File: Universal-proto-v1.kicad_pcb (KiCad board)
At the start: 2 copper layers, 2 parts, among them J1 Bus_ISA_8bit, U1 RP2350B

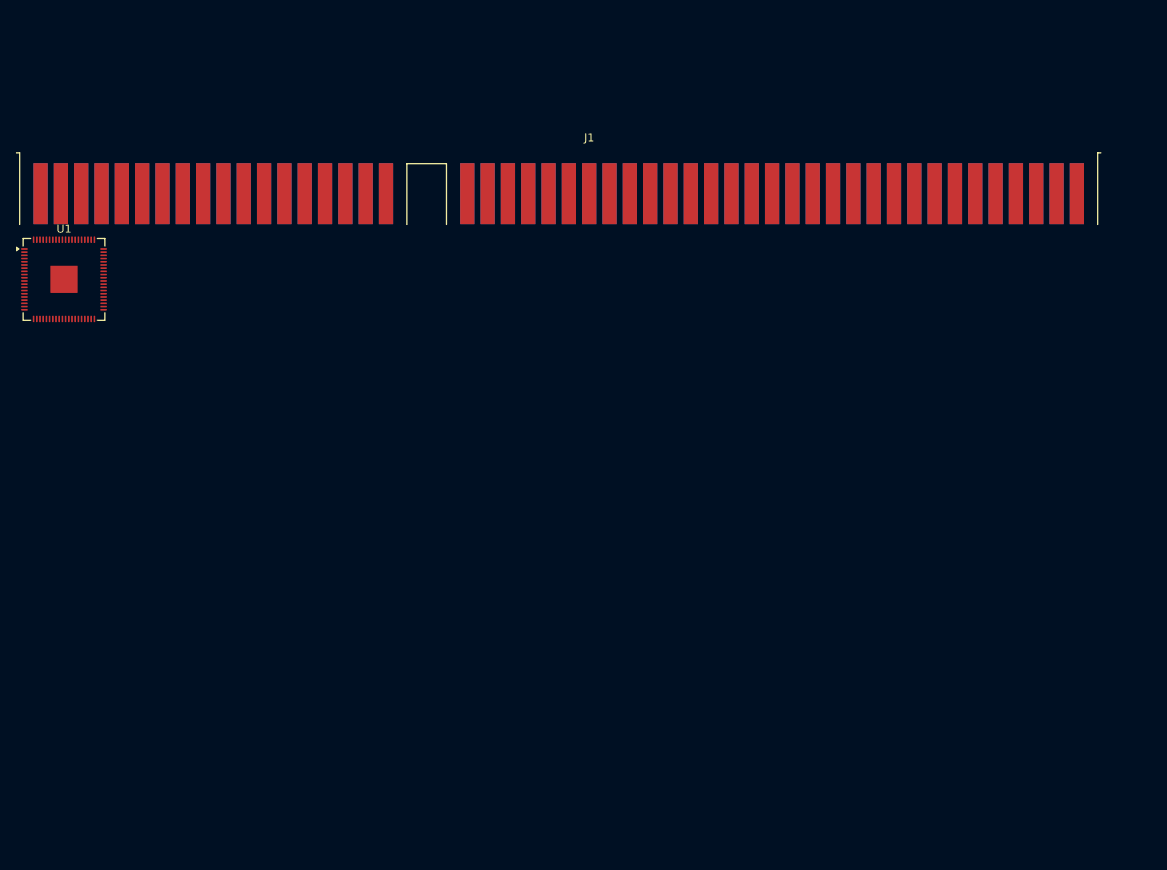
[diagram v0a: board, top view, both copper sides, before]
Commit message: Start work on PCB
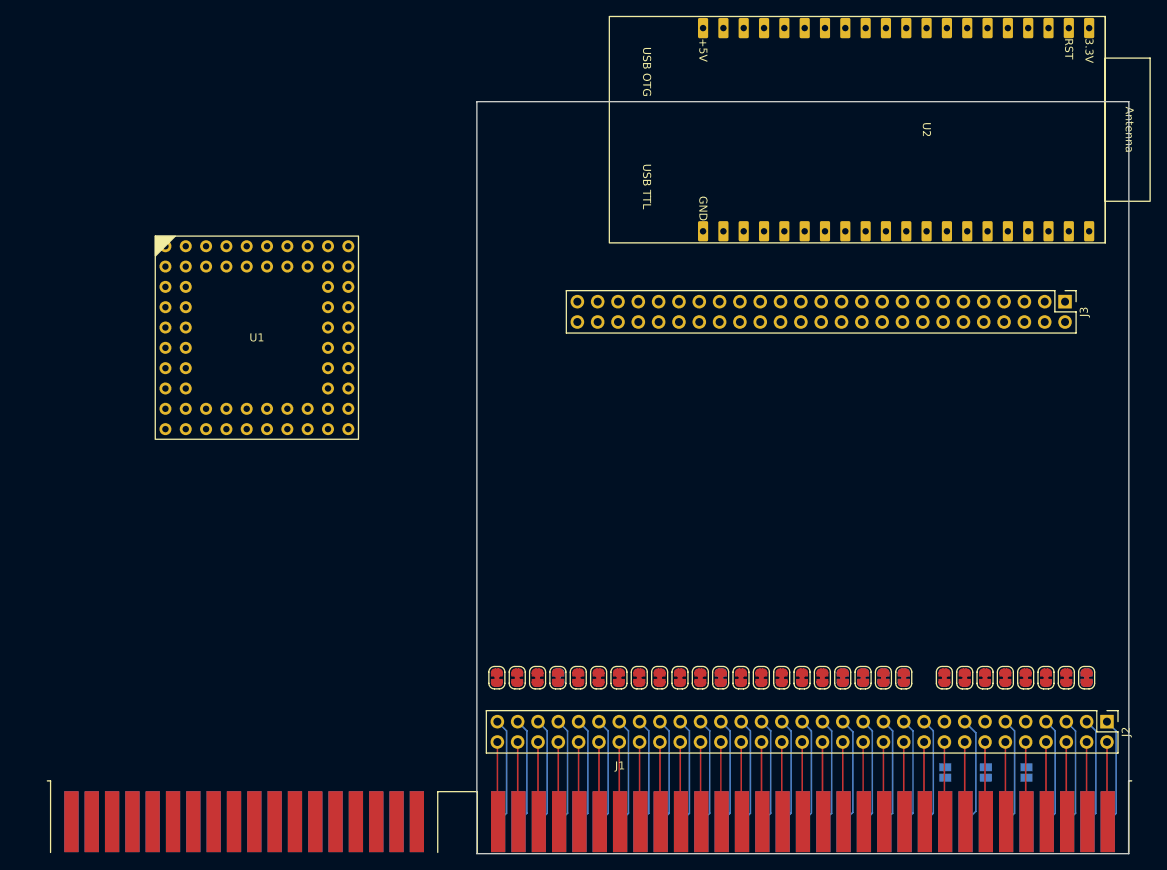
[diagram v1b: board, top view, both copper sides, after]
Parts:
- added J2: ISA Breakout, Connector_PinHeader_2.54mm:PinHeader_2x31_P2.54mm_Vertical, F.Cu at (185.8, 127.5)
- added J3: Pico GPIO Breakout, Connector_PinHeader_2.54mm:PinHeader_2x25_P2.54mm_Vertical, F.Cu at (180.5, 75.0)
- added JP1: SolderJumper_2_Bridged, Jumper:SolderJumper-2_P1.3mm_Bridged_RoundedPad1.0x1.5mm, F.Cu at (109.5, 122.0)
- added JP10: SolderJumper_2_Bridged, Jumper:SolderJumper-2_P1.3mm_Bridged_RoundedPad1.0x1.5mm, F.Cu at (132.4, 122.0)
- added JP11: SolderJumper_2_Bridged, Jumper:SolderJumper-2_P1.3mm_Bridged_RoundedPad1.0x1.5mm, F.Cu at (134.9, 122.0)
- added JP12: SolderJumper_2_Bridged, Jumper:SolderJumper-2_P1.3mm_Bridged_RoundedPad1.0x1.5mm, F.Cu at (137.5, 122.0)
- added JP13: SolderJumper_2_Bridged, Jumper:SolderJumper-2_P1.3mm_Bridged_RoundedPad1.0x1.5mm, F.Cu at (140.0, 122.0)
- added JP14: SolderJumper_2_Bridged, Jumper:SolderJumper-2_P1.3mm_Bridged_RoundedPad1.0x1.5mm, F.Cu at (142.6, 122.0)
- added JP15: SolderJumper_2_Bridged, Jumper:SolderJumper-2_P1.3mm_Bridged_RoundedPad1.0x1.5mm, F.Cu at (145.1, 122.0)
- added JP16: SolderJumper_2_Bridged, Jumper:SolderJumper-2_P1.3mm_Bridged_RoundedPad1.0x1.5mm, F.Cu at (147.6, 122.0)
- added JP17: SolderJumper_2_Bridged, Jumper:SolderJumper-2_P1.3mm_Bridged_RoundedPad1.0x1.5mm, F.Cu at (150.2, 122.0)
- added JP18: SolderJumper_2_Bridged, Jumper:SolderJumper-2_P1.3mm_Bridged_RoundedPad1.0x1.5mm, F.Cu at (152.7, 122.0)
- added JP19: SolderJumper_2_Bridged, Jumper:SolderJumper-2_P1.3mm_Bridged_RoundedPad1.0x1.5mm, F.Cu at (155.3, 122.0)
- added JP2: SolderJumper_2_Bridged, Jumper:SolderJumper-2_P1.3mm_Bridged_RoundedPad1.0x1.5mm, F.Cu at (112.0, 122.0)
- added JP20: SolderJumper_2_Bridged, Jumper:SolderJumper-2_P1.3mm_Bridged_RoundedPad1.0x1.5mm, F.Cu at (157.8, 122.0)
- added JP21: SolderJumper_2_Bridged, Jumper:SolderJumper-2_P1.3mm_Bridged_RoundedPad1.0x1.5mm, F.Cu at (165.4, 122.0)
- added JP22: SolderJumper_2_Bridged, Jumper:SolderJumper-2_P1.3mm_Bridged_RoundedPad1.0x1.5mm, F.Cu at (168.0, 122.0)
- added JP23: SolderJumper_2_Bridged, Jumper:SolderJumper-2_P1.3mm_Bridged_RoundedPad1.0x1.5mm, F.Cu at (170.5, 122.0)
- added JP24: SolderJumper_2_Bridged, Jumper:SolderJumper-2_P1.3mm_Bridged_RoundedPad1.0x1.5mm, F.Cu at (173.1, 122.0)
- added JP25: SolderJumper_2_Bridged, Jumper:SolderJumper-2_P1.3mm_Bridged_RoundedPad1.0x1.5mm, F.Cu at (175.6, 122.0)
- added JP26: SolderJumper_2_Bridged, Jumper:SolderJumper-2_P1.3mm_Bridged_RoundedPad1.0x1.5mm, F.Cu at (178.1, 122.0)
- added JP27: SolderJumper_2_Bridged, Jumper:SolderJumper-2_P1.3mm_Bridged_RoundedPad1.0x1.5mm, F.Cu at (180.7, 122.0)
- added JP28: SolderJumper_2_Bridged, Jumper:SolderJumper-2_P1.3mm_Bridged_RoundedPad1.0x1.5mm, F.Cu at (183.2, 122.0)
- added JP29: SolderJumper_2_Bridged, Jumper:SolderJumper-2_P1.3mm_Bridged_RoundedPad1.0x1.5mm, B.Cu at (157.8, 122.0)
- added JP3: SolderJumper_2_Bridged, Jumper:SolderJumper-2_P1.3mm_Bridged_RoundedPad1.0x1.5mm, F.Cu at (114.6, 122.0)
- added JP30: SolderJumper_2_Bridged, Jumper:SolderJumper-2_P1.3mm_Bridged_RoundedPad1.0x1.5mm, B.Cu at (160.4, 122.0)
- added JP31: SolderJumper_2_Bridged, Jumper:SolderJumper-2_P1.3mm_Bridged_RoundedPad1.0x1.5mm, B.Cu at (152.7, 122.0)
- added JP32: SolderJumper_2_Bridged, Jumper:SolderJumper-2_P1.3mm_Bridged_RoundedPad1.0x1.5mm, B.Cu at (155.3, 122.0)
- added JP33: SolderJumper_2_Bridged, Jumper:SolderJumper-2_P1.3mm_Bridged_RoundedPad1.0x1.5mm, F.Cu at (160.4, 122.0)
- added JP34: SolderJumper_2_Bridged, Jumper:SolderJumper-2_P1.3mm_Bridged_RoundedPad1.0x1.5mm, B.Cu at (137.5, 122.0)
- added JP35: SolderJumper_2_Bridged, Jumper:SolderJumper-2_P1.3mm_Bridged_RoundedPad1.0x1.5mm, B.Cu at (117.2, 122.0)
- added JP36: SolderJumper_2_Bridged, Jumper:SolderJumper-2_P1.3mm_Bridged_RoundedPad1.0x1.5mm, B.Cu at (183.2, 122.0)
- added JP37: SolderJumper_2_Open, Jumper:SolderJumper-2_P1.3mm_Open_Pad1.0x1.5mm, B.Cu at (165.5, 133.8)
- added JP38: SolderJumper_2_Open, Jumper:SolderJumper-2_P1.3mm_Open_Pad1.0x1.5mm, B.Cu at (170.6, 133.8)
- added JP39: SolderJumper_2_Open, Jumper:SolderJumper-2_P1.3mm_Open_Pad1.0x1.5mm, B.Cu at (175.7, 133.8)
- added JP4: SolderJumper_2_Bridged, Jumper:SolderJumper-2_P1.3mm_Bridged_RoundedPad1.0x1.5mm, F.Cu at (117.1, 122.0)
- added JP5: SolderJumper_2_Bridged, Jumper:SolderJumper-2_P1.3mm_Bridged_RoundedPad1.0x1.5mm, F.Cu at (119.7, 122.0)
- added JP6: SolderJumper_2_Bridged, Jumper:SolderJumper-2_P1.3mm_Bridged_RoundedPad1.0x1.5mm, F.Cu at (122.2, 122.0)
- added JP7: SolderJumper_2_Bridged, Jumper:SolderJumper-2_P1.3mm_Bridged_RoundedPad1.0x1.5mm, F.Cu at (124.8, 122.0)
- added JP8: SolderJumper_2_Bridged, Jumper:SolderJumper-2_P1.3mm_Bridged_RoundedPad1.0x1.5mm, F.Cu at (127.3, 122.0)
- added JP9: SolderJumper_2_Bridged, Jumper:SolderJumper-2_P1.3mm_Bridged_RoundedPad1.0x1.5mm, F.Cu at (129.8, 122.0)
- added U2: ~, FujiNet:ESP32-S3-CAM, F.Cu at (183.5, 40.8)
- U1: value RP2350B -> ~; footprint Package_DFN_QFN:QFN-80-1EP_10x10mm_P0.4mm_EP3.4x3.4mm -> FujiNet:WaveShare-Core-RP2350B
- moved J1 78.6 mm to (185.9, 140.0)
- moved U1 35.5 mm to (90.9, 71.9)
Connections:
- J1 pad 1: unconnected-(J1-GND-Pad1) -> /GND
- J1 pad 10: unconnected-(J1-GND-Pad10) -> /GND
- J1 pad 11: unconnected-(J1-~{SMEMW}-Pad11) -> /~{SMEMW}
- J1 pad 12: unconnected-(J1-~{SMEMR}-Pad12) -> /~{SMEMR}
- J1 pad 13: unconnected-(J1-~{IOW}-Pad13) -> /~{IOW}
- J1 pad 14: unconnected-(J1-~{IOR}-Pad14) -> /~{IOR}
- J1 pad 15: unconnected-(J1-~{DACK3}-Pad15) -> /~{DACK3}
- J1 pad 16: unconnected-(J1-DRQ3-Pad16) -> /DRQ3
- J1 pad 17: unconnected-(J1-~{DACK1}-Pad17) -> /~{DACK1}
- J1 pad 18: unconnected-(J1-DRQ1-Pad18) -> /DRQ1
- J1 pad 19: unconnected-(J1-~{DACK0}-Pad19) -> /~{DACK0}
- J1 pad 2: unconnected-(J1-RESET-Pad2) -> /RESET
- J1 pad 20: unconnected-(J1-CLK-Pad20) -> /CLK
- J1 pad 21: unconnected-(J1-IRQ7-Pad21) -> /IRQ7
- J1 pad 22: unconnected-(J1-IRQ6-Pad22) -> /IRQ6
- J1 pad 23: unconnected-(J1-IRQ5-Pad23) -> /IRQ5
- J1 pad 24: unconnected-(J1-IRQ4-Pad24) -> /IRQ4
- J1 pad 25: unconnected-(J1-IRQ3-Pad25) -> /IRQ3
- J1 pad 26: unconnected-(J1-~{DACK2}-Pad26) -> /~{DACK2}
- J1 pad 27: unconnected-(J1-TC-Pad27) -> /TC
- J1 pad 28: unconnected-(J1-ALE-Pad28) -> /ALE
- J1 pad 29: unconnected-(J1-VCC-Pad29) -> /VCC
- J1 pad 3: unconnected-(J1-VCC-Pad3) -> /VCC
- J1 pad 30: unconnected-(J1-OSC-Pad30) -> /OSC
- J1 pad 31: unconnected-(J1-GND-Pad31) -> /GND
- J1 pad 32: unconnected-(J1-IO-Pad32) -> /IO
- J1 pad 33: unconnected-(J1-DB7-Pad33) -> /DB7
- J1 pad 34: unconnected-(J1-DB6-Pad34) -> /DB6
- J1 pad 35: unconnected-(J1-DB5-Pad35) -> /DB5
- J1 pad 36: unconnected-(J1-DB4-Pad36) -> /DB4
- J1 pad 37: unconnected-(J1-DB3-Pad37) -> /DB3
- J1 pad 38: unconnected-(J1-DB2-Pad38) -> /DB2
- J1 pad 39: unconnected-(J1-DB1-Pad39) -> /DB1
- J1 pad 4: unconnected-(J1-IRQ2-Pad4) -> /IRQ2
- J1 pad 40: unconnected-(J1-DB0-Pad40) -> /DB0
- J1 pad 41: unconnected-(J1-IO_READY-Pad41) -> /IO_READY
- J1 pad 42: unconnected-(J1-AEN-Pad42) -> /AEN
- J1 pad 43: unconnected-(J1-BA19-Pad43) -> /BA19
- J1 pad 44: unconnected-(J1-BA18-Pad44) -> /BA18
- J1 pad 45: unconnected-(J1-BA17-Pad45) -> /BA17
- J1 pad 46: unconnected-(J1-BA16-Pad46) -> /BA16
- J1 pad 47: unconnected-(J1-BA15-Pad47) -> /BA15
- J1 pad 48: unconnected-(J1-BA14-Pad48) -> /BA14
- J1 pad 49: unconnected-(J1-BA13-Pad49) -> /BA13
- J1 pad 5: unconnected-(J1--5V-Pad5) -> /ISA_-5V
- J1 pad 50: unconnected-(J1-BA12-Pad50) -> /BA12
- J1 pad 51: unconnected-(J1-BA11-Pad51) -> /BA11
- J1 pad 52: unconnected-(J1-BA10-Pad52) -> /BA10
- J1 pad 53: unconnected-(J1-BA09-Pad53) -> /BA09
- J1 pad 54: unconnected-(J1-BA08-Pad54) -> /BA08
- J1 pad 55: unconnected-(J1-BA07-Pad55) -> /BA07
- J1 pad 56: unconnected-(J1-BA06-Pad56) -> /BA06
- J1 pad 57: unconnected-(J1-BA05-Pad57) -> /BA05
- J1 pad 58: unconnected-(J1-BA04-Pad58) -> /BA04
- J1 pad 59: unconnected-(J1-BA03-Pad59) -> /BA03
- J1 pad 6: unconnected-(J1-DRQ2-Pad6) -> /DRQ2
- J1 pad 60: unconnected-(J1-BA02-Pad60) -> /BA02
- J1 pad 61: unconnected-(J1-BA01-Pad61) -> /BA01
- J1 pad 62: unconnected-(J1-BA00-Pad62) -> /BA00
- J1 pad 7: unconnected-(J1--12V-Pad7) -> /ISA_-12V
- J1 pad 8: unconnected-(J1-UNUSED-Pad8) -> /UNUSED
- J1 pad 9: unconnected-(J1-+12V-Pad9) -> /ISA_+12V
- U1 pad 1: unconnected-(U1-GPIO4-Pad1) -> /GP1_ISA_A1
- U1 pad 10: Net-(U1-DVDD-Pad10) -> /GP10_ISA_A10
- U1 pad 11: unconnected-(U1-GPIO12-Pad11) -> /GP11_ISA_A11
- U1 pad 12: unconnected-(U1-GPIO13-Pad12) -> /GP12_ISA_A12
- U1 pad 13: unconnected-(U1-GPIO14-Pad13) -> /GP13_ISA_A13
- U1 pad 14: unconnected-(U1-GPIO15-Pad14) -> /GP14_ISA_A14
- U1 pad 15: Net-(U1-IOVDD-Pad15) -> /GP15_ISA_A15
- U1 pad 16: unconnected-(U1-GPIO16-Pad16) -> /GP16_ISA_A16
- U1 pad 17: unconnected-(U1-GPIO17-Pad17) -> /GP17_ISA_A17
- U1 pad 18: unconnected-(U1-GPIO18-Pad18) -> /GP18_ISA_A18
- U1 pad 19: unconnected-(U1-GPIO19-Pad19) -> /GP19_ISA_A19
- U1 pad 2: unconnected-(U1-GPIO5-Pad2) -> /GP2_ISA_A2
- U1 pad 20: unconnected-(U1-GPIO20-Pad20) -> /GP20_ISA_D0
- U1 pad 21: unconnected-(U1-GPIO21-Pad21) -> /GP21_ISA_D1
- U1 pad 22: unconnected-(U1-GPIO22-Pad22) -> /GP22_ISA_D2
- U1 pad 23: unconnected-(U1-GPIO23-Pad23) -> /GP23_ISA_D3
- U1 pad 24: Net-(U1-IOVDD-Pad15) -> /GP24_ISA_D4
- U1 pad 25: unconnected-(U1-GPIO24-Pad25) -> /GP25_ISA_D5
- U1 pad 26: unconnected-(U1-GPIO25-Pad26) -> /GP26_ISA_D6
- U1 pad 27: unconnected-(U1-GPIO26-Pad27) -> /GP27_ISA_D7
- U1 pad 28: unconnected-(U1-GPIO27-Pad28) -> /GP28_ISA_MEMR
- U1 pad 29: Net-(U1-IOVDD-Pad15) -> /GP29_ISA_MEMW
- U1 pad 3: unconnected-(U1-GPIO6-Pad3) -> /GP3_ISA_A3
- U1 pad 30: unconnected-(U1-XIN-Pad30) -> /GP30_ISA_IOR
- U1 pad 31: unconnected-(U1-XOUT-Pad31) -> /GP31_ISA_IOW
- U1 pad 32: Net-(U1-DVDD-Pad10) -> /GP32_ISA_AEN
- U1 pad 33: unconnected-(U1-SWCLK-Pad33) -> /GP33_ISA_CLK
- U1 pad 34: unconnected-(U1-SWDIO-Pad34) -> /GP34_ISA_ALE
- U1 pad 35: unconnected-(U1-RUN-Pad35) -> /GP35_ISA_RESET
- U1 pad 36: unconnected-(U1-GPIO28-Pad36) -> /GP36
- U1 pad 37: unconnected-(U1-GPIO29-Pad37) -> /GP37
- U1 pad 38: unconnected-(U1-GPIO30-Pad38) -> /GP38
- U1 pad 39: unconnected-(U1-GPIO31-Pad39) -> /GP39
- U1 pad 4: unconnected-(U1-GPIO7-Pad4) -> /GP4_ISA_A4
- U1 pad 40: unconnected-(U1-GPIO32-Pad40) -> /GP40
- U1 pad 41: Net-(U1-IOVDD-Pad15) -> /GP41
- U1 pad 42: unconnected-(U1-GPIO33-Pad42) -> /GP42
- U1 pad 43: unconnected-(U1-GPIO34-Pad43) -> /GP43
- U1 pad 44: unconnected-(U1-GPIO35-Pad44) -> /GP44
- U1 pad 45: unconnected-(U1-GPIO36-Pad45) -> /GP45
- U1 pad 46: unconnected-(U1-GPIO37-Pad46) -> /GP46
- U1 pad 47: unconnected-(U1-GPIO38-Pad47) -> /GP47
- U1 pad 5: Net-(U1-IOVDD-Pad15) -> /GP5_ISA_A5
- U1 pad 6: unconnected-(U1-GPIO8-Pad6) -> /GP6_ISA_A6
- U1 pad 7: unconnected-(U1-GPIO9-Pad7) -> /GP7_ISA_A7
- U1 pad 8: unconnected-(U1-GPIO10-Pad8) -> /GP8_ISA_A8
- U1 pad 9: unconnected-(U1-GPIO11-Pad9) -> /GP9_ISA_A9
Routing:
- net /GND: track 0.00 -> 40.2 mm
- net /VCC: track 0.00 -> 26.8 mm
- net /UNUSED: track 0.00 -> 13.6 mm
- net /~{IOR}: track 0.00 -> 13.5 mm
- net /~{SMEMR}: track 0.00 -> 13.4 mm
- net /~{IOW}: track 0.00 -> 13.4 mm
- net /~{DACK0}: track 0.00 -> 13.4 mm
- net /RESET: track 0.00 -> 13.4 mm
- net /IRQ5: track 0.00 -> 13.4 mm
- net /IRQ4: track 0.00 -> 13.4 mm
- net /DRQ3: track 0.00 -> 13.4 mm
- net /DRQ2: track 0.00 -> 13.4 mm
- net /CLK: track 0.00 -> 13.4 mm
- net /OSC: track 0.00 -> 13.4 mm
- net /~{DACK3}: track 0.00 -> 13.4 mm
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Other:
- board outline added: 81.5 x 94 mm
